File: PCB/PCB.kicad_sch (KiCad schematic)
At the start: 13 parts, among them SW1 RotaryEncoder_Switch, SW2 RotaryEncoder_Switch, SW3 SW_Push, SW4 SW_Push, SW5 SW_Push, SW6 SW_Push, U1 XIAO-RP2040-DIP

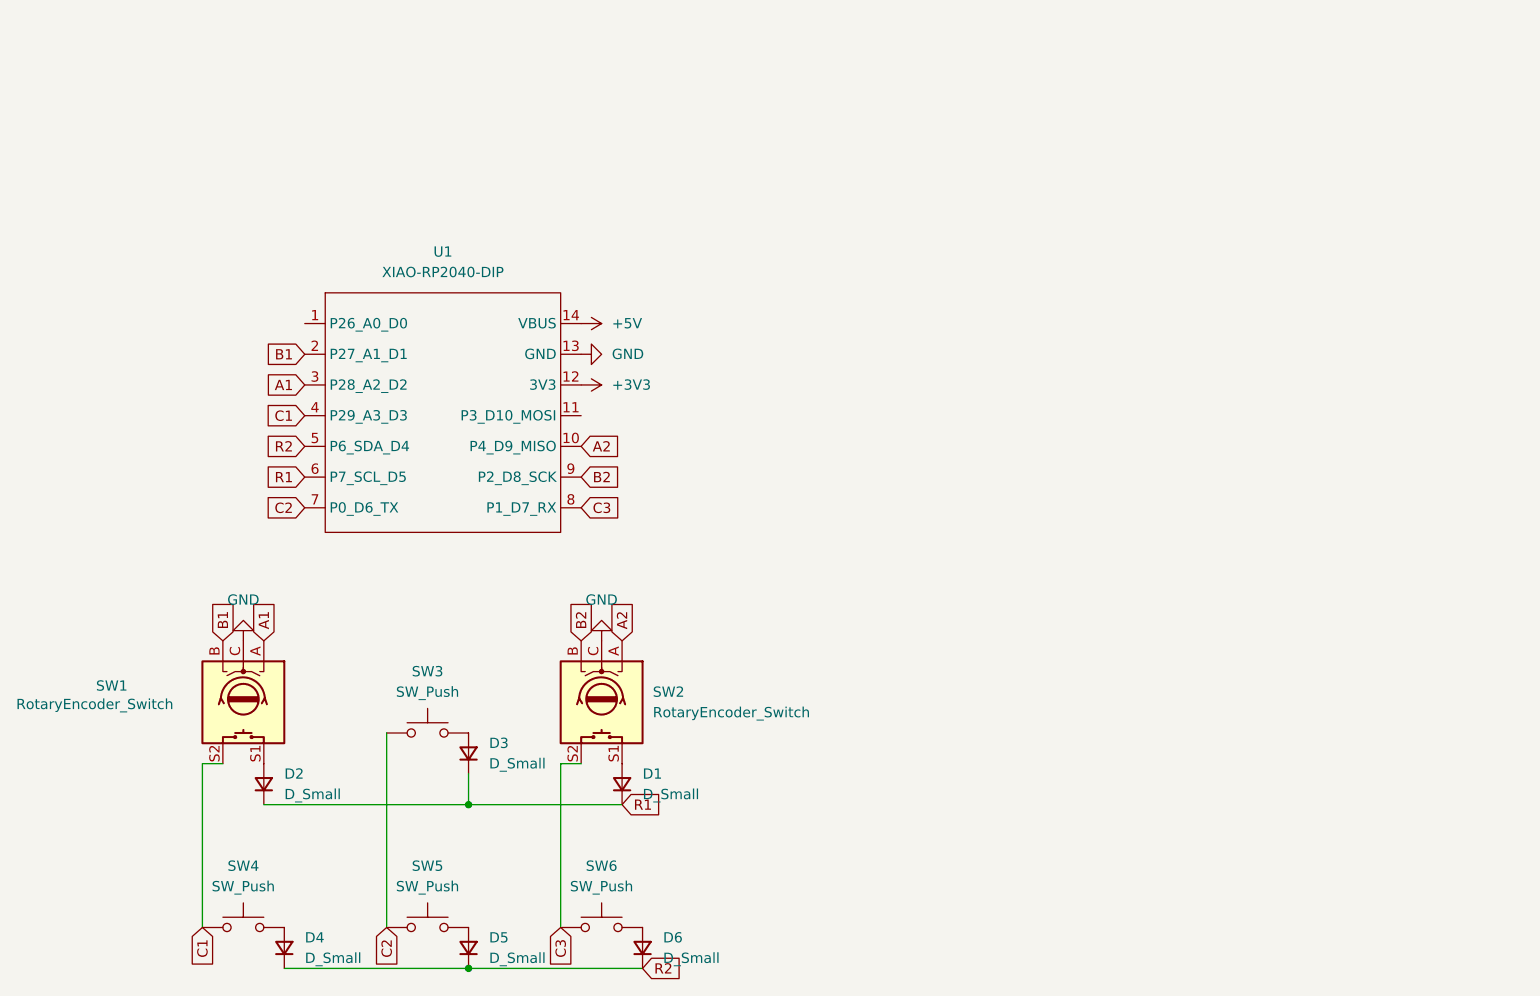
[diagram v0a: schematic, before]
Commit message: bleh
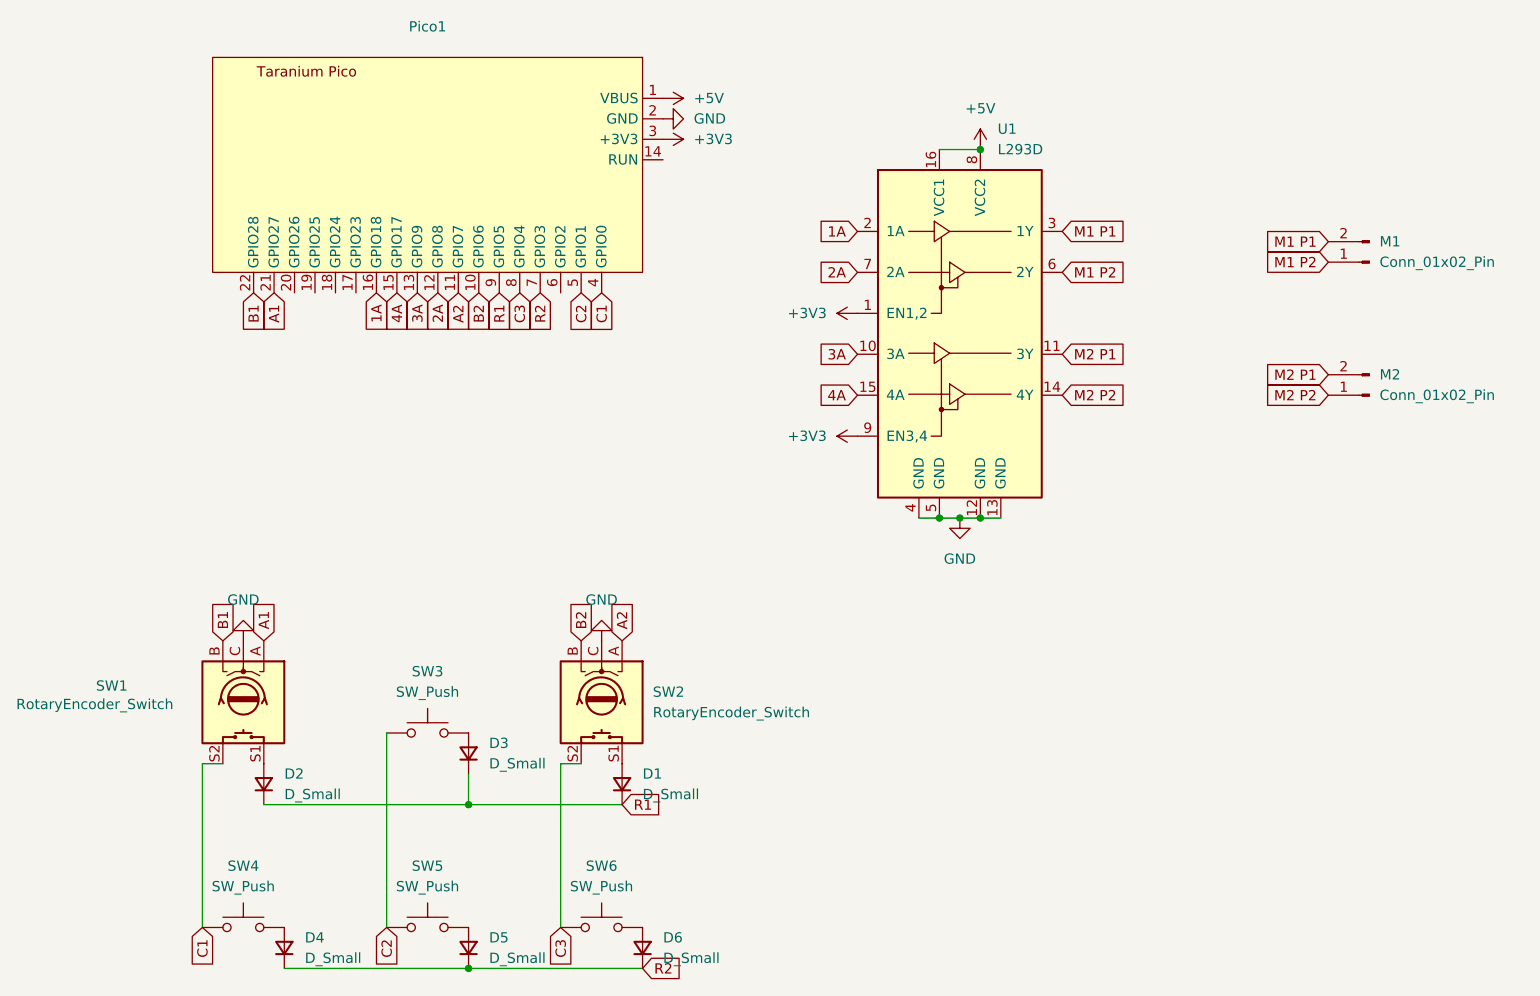
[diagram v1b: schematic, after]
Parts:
- removed U1: XIAO-RP2040-DIP, Taranium-libs:XIAO-RP2040-DIP, symbol Seeed_Studio_XIAO_Series:XIAO-RP2040-DIP
- added M1, M2: Conn_01x02_Pin, Connector_PinHeader_2.54mm:PinHeader_1x02_P2.54mm_Vertical, symbol Connector:Conn_01x02_Pin
- added Pico1: ~, Taranium-libs:Taranium_Pico, symbol Taranium-libs:Taranium_Pico
- added U1: L293D, Package_DIP:DIP-16_W7.62mm, symbol Driver_Motor:L293D
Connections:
- net +3V3: now also Pico1.3 (+3V3), U1.1 (EN1,2), U1.9 (EN3,4)
- net +5V: now also Pico1.1 (VBUS), U1.16 (VCC1), U1.8 (VCC2)
- net A1: now also Pico1.21 (GPIO27)
- net A2: now also Pico1.11 (GPIO7)
- net B1: now also Pico1.22 (GPIO28)
- net B2: now also Pico1.10 (GPIO6)
- net C1: now also Pico1.4 (GPIO0)
- net C2: now also Pico1.5 (GPIO1)
- net C3: now also Pico1.8 (GPIO4)
- net GND: now also Pico1.2 (GND), U1.12 (GND), U1.13 (GND), U1.4 (GND), U1.5 (GND)
- net R1: now also Pico1.9 (GPIO5)
- net R2: now also Pico1.7 (GPIO3)
- new net 1A: Pico1.16 (GPIO18), U1.2 (1A)
- new net 2A: Pico1.12 (GPIO8), U1.7 (2A)
- new net 3A: Pico1.13 (GPIO9), U1.10 (3A)
- new net 4A: Pico1.15 (GPIO17), U1.15 (4A)
- new net M1 P1: M1.2 (Pin_2), U1.3 (1Y)
- new net M1 P2: M1.1 (Pin_1), U1.6 (2Y)
- new net M2 P1: M2.2 (Pin_2), U1.11 (3Y)
- new net M2 P2: M2.1 (Pin_1), U1.14 (4Y)
